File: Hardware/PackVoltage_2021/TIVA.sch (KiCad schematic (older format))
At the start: 1 part, among them U24 TM4C129E_Launchpad

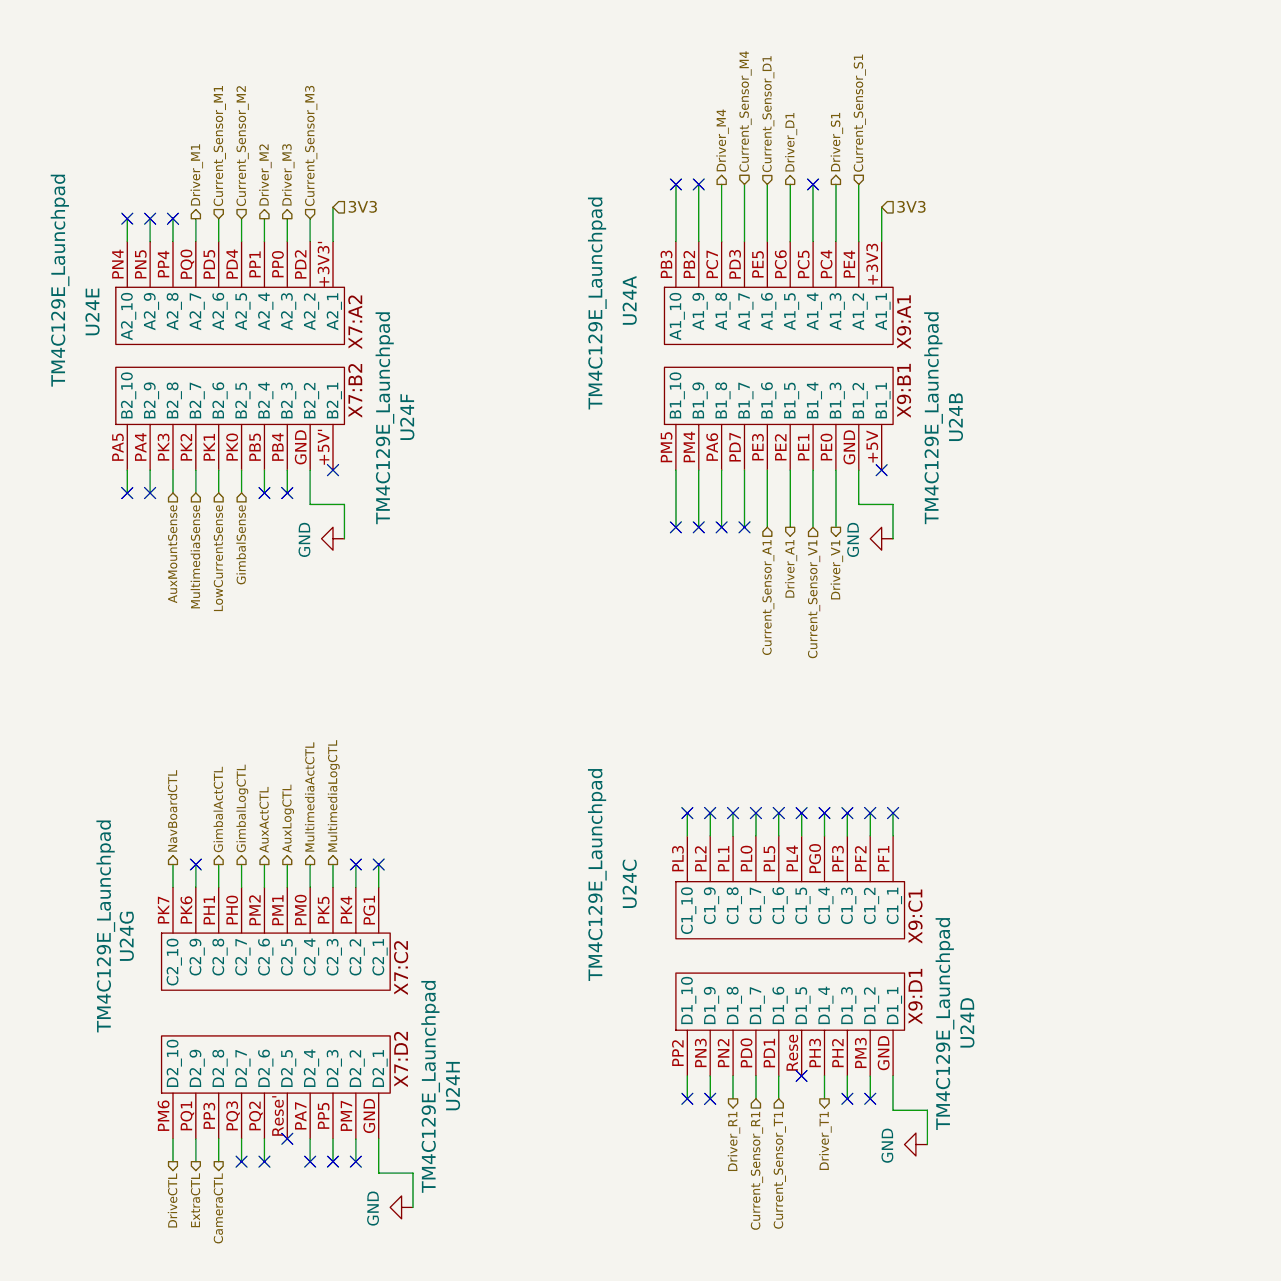
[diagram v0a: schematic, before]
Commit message: netlist
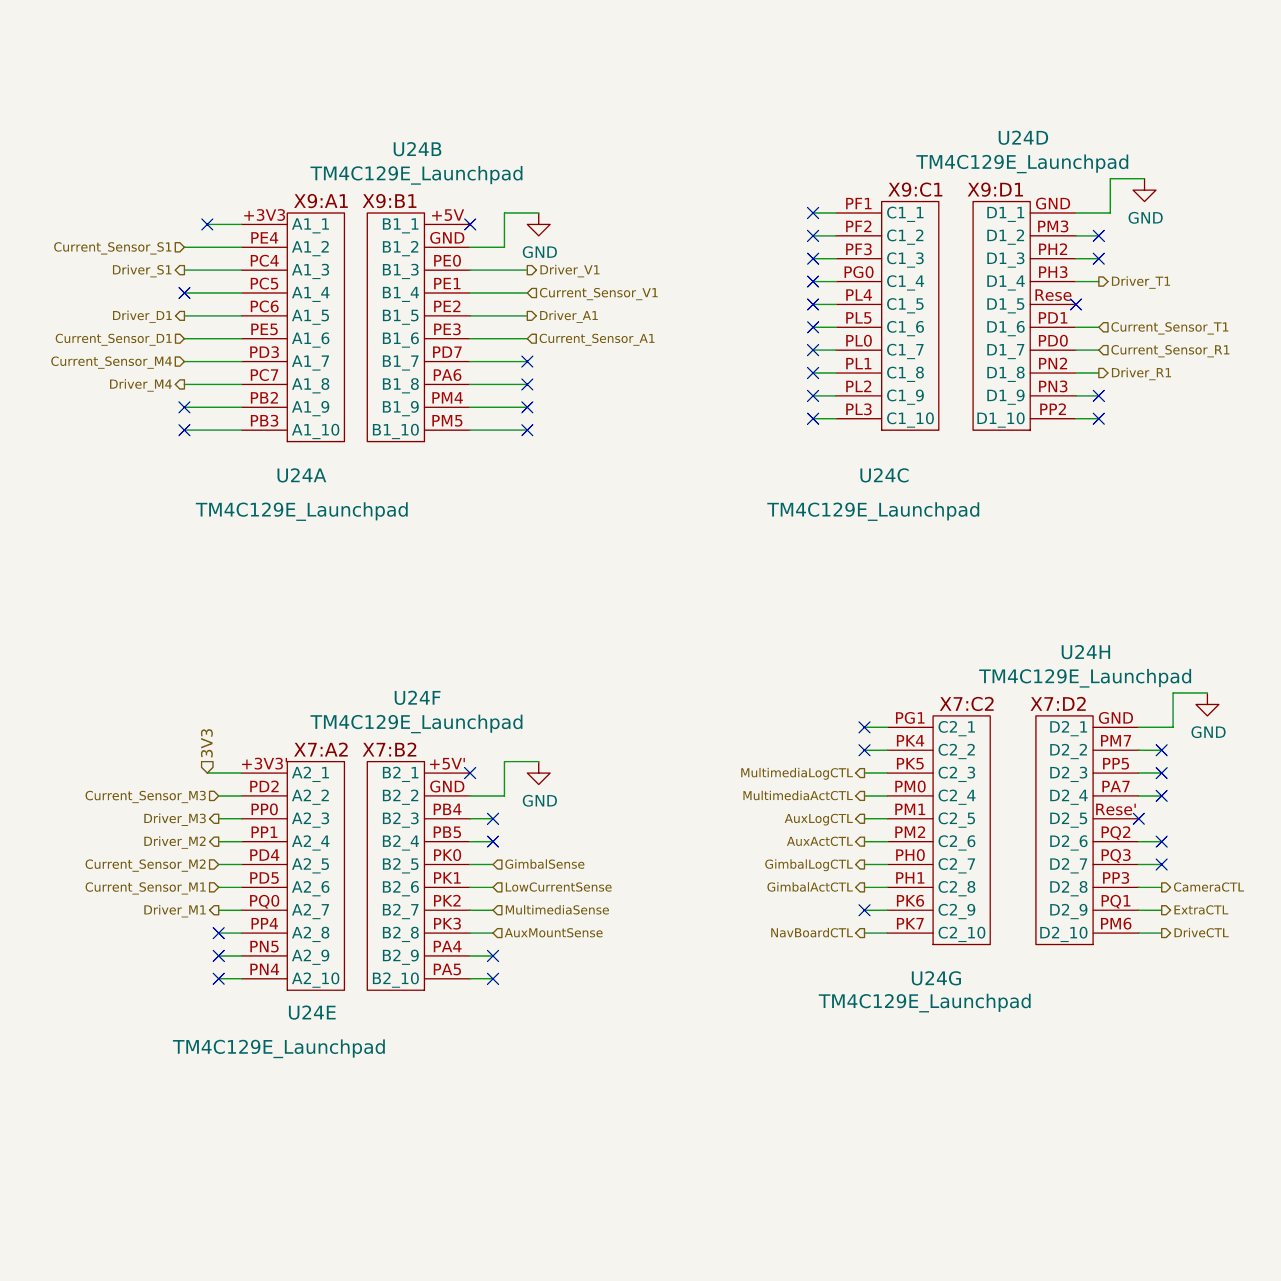
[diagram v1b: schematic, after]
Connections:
- net 3V3: no longer U24.+3V3 (A1_1)
- no-connect marks 40 -> 41
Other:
- moved on the sheet: U24A, U24B, U24C, U24D, U24E, U24F, U24G, U24H

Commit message: Revert "netlist"
This reverts commit 1af6446f6858f10edba603e339066d14f3a2f95b.
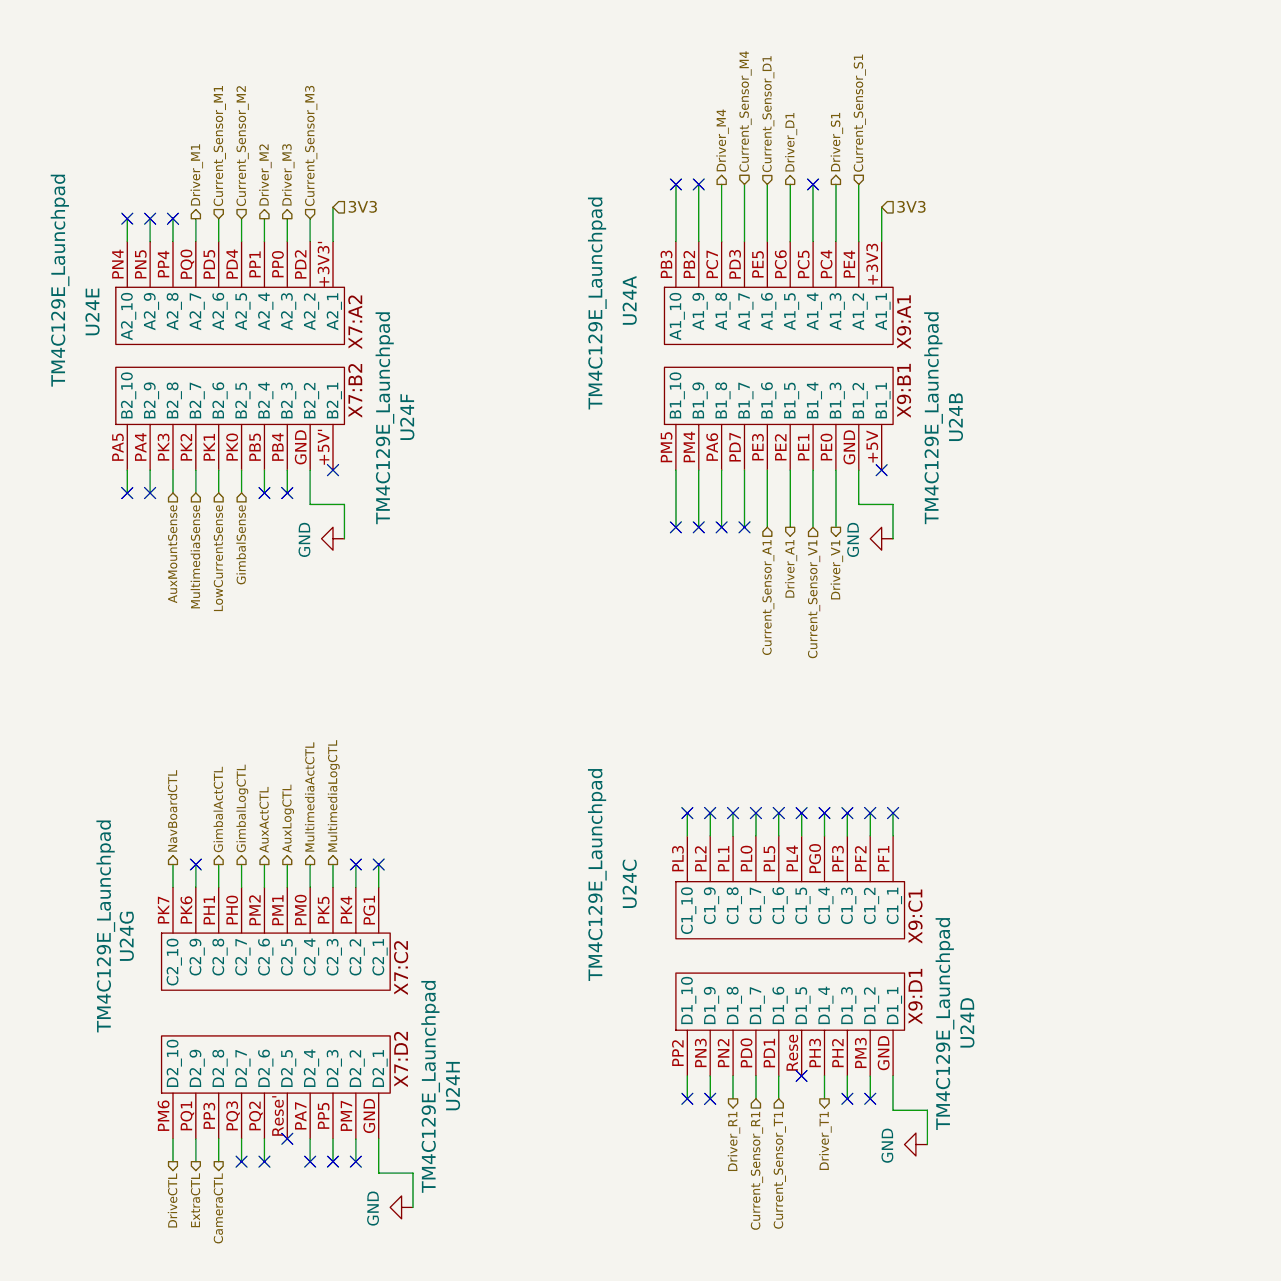
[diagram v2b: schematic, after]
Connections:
- net 3V3: now also U24.+3V3 (A1_1)
- no-connect marks 41 -> 40
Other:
- moved on the sheet: U24A, U24B, U24C, U24D, U24E, U24F, U24G, U24H
